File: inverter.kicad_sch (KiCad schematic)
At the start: 38 parts, among them IC3 L6498D, IC4 L6498D, IC5 L6498D, J2 43650-0303, J5 2159310271, Q1 IPD320N20N3GATMA1, Q2 IPD320N20N3GATMA1, Q3 IPD320N20N3GATMA1, Q4 IPD320N20N3GATMA1, Q5 IPD320N20N3GATMA1, Q6 IPD320N20N3GATMA1

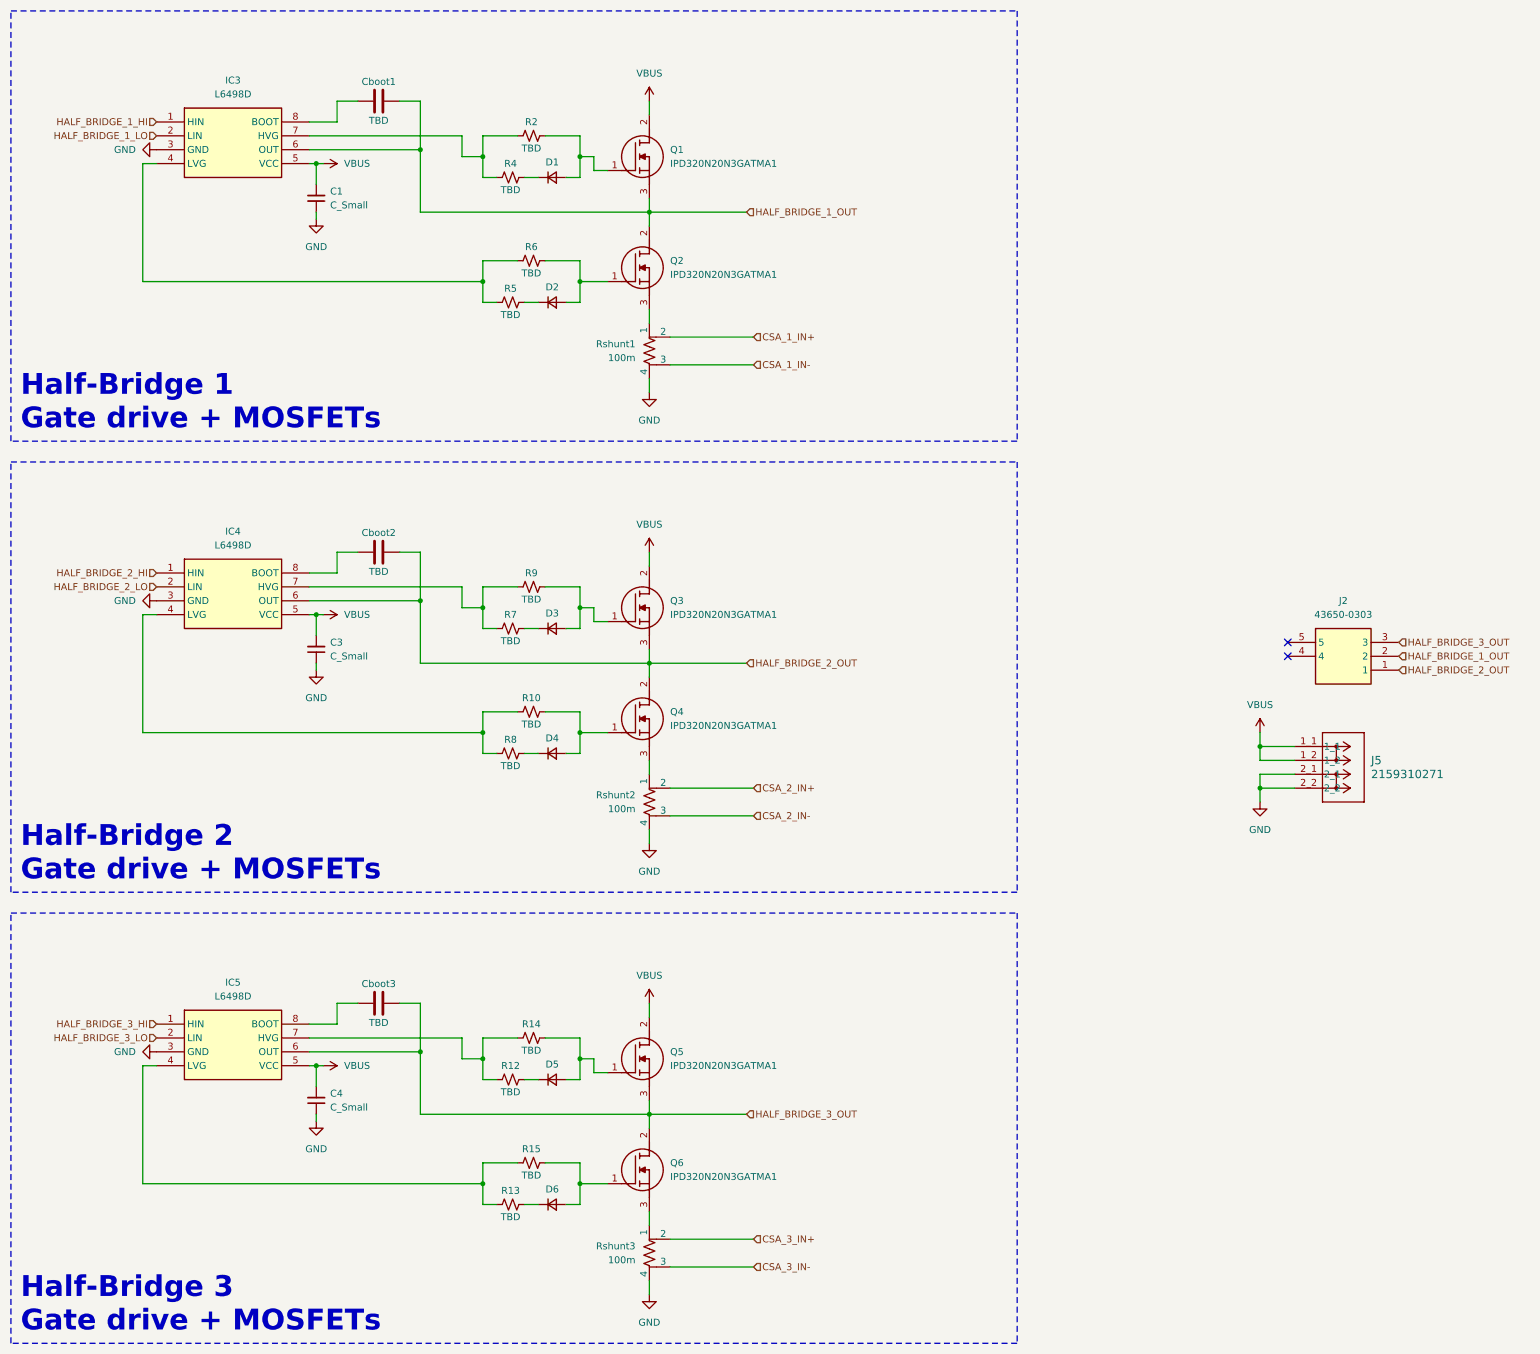
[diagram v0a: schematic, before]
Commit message: More routing
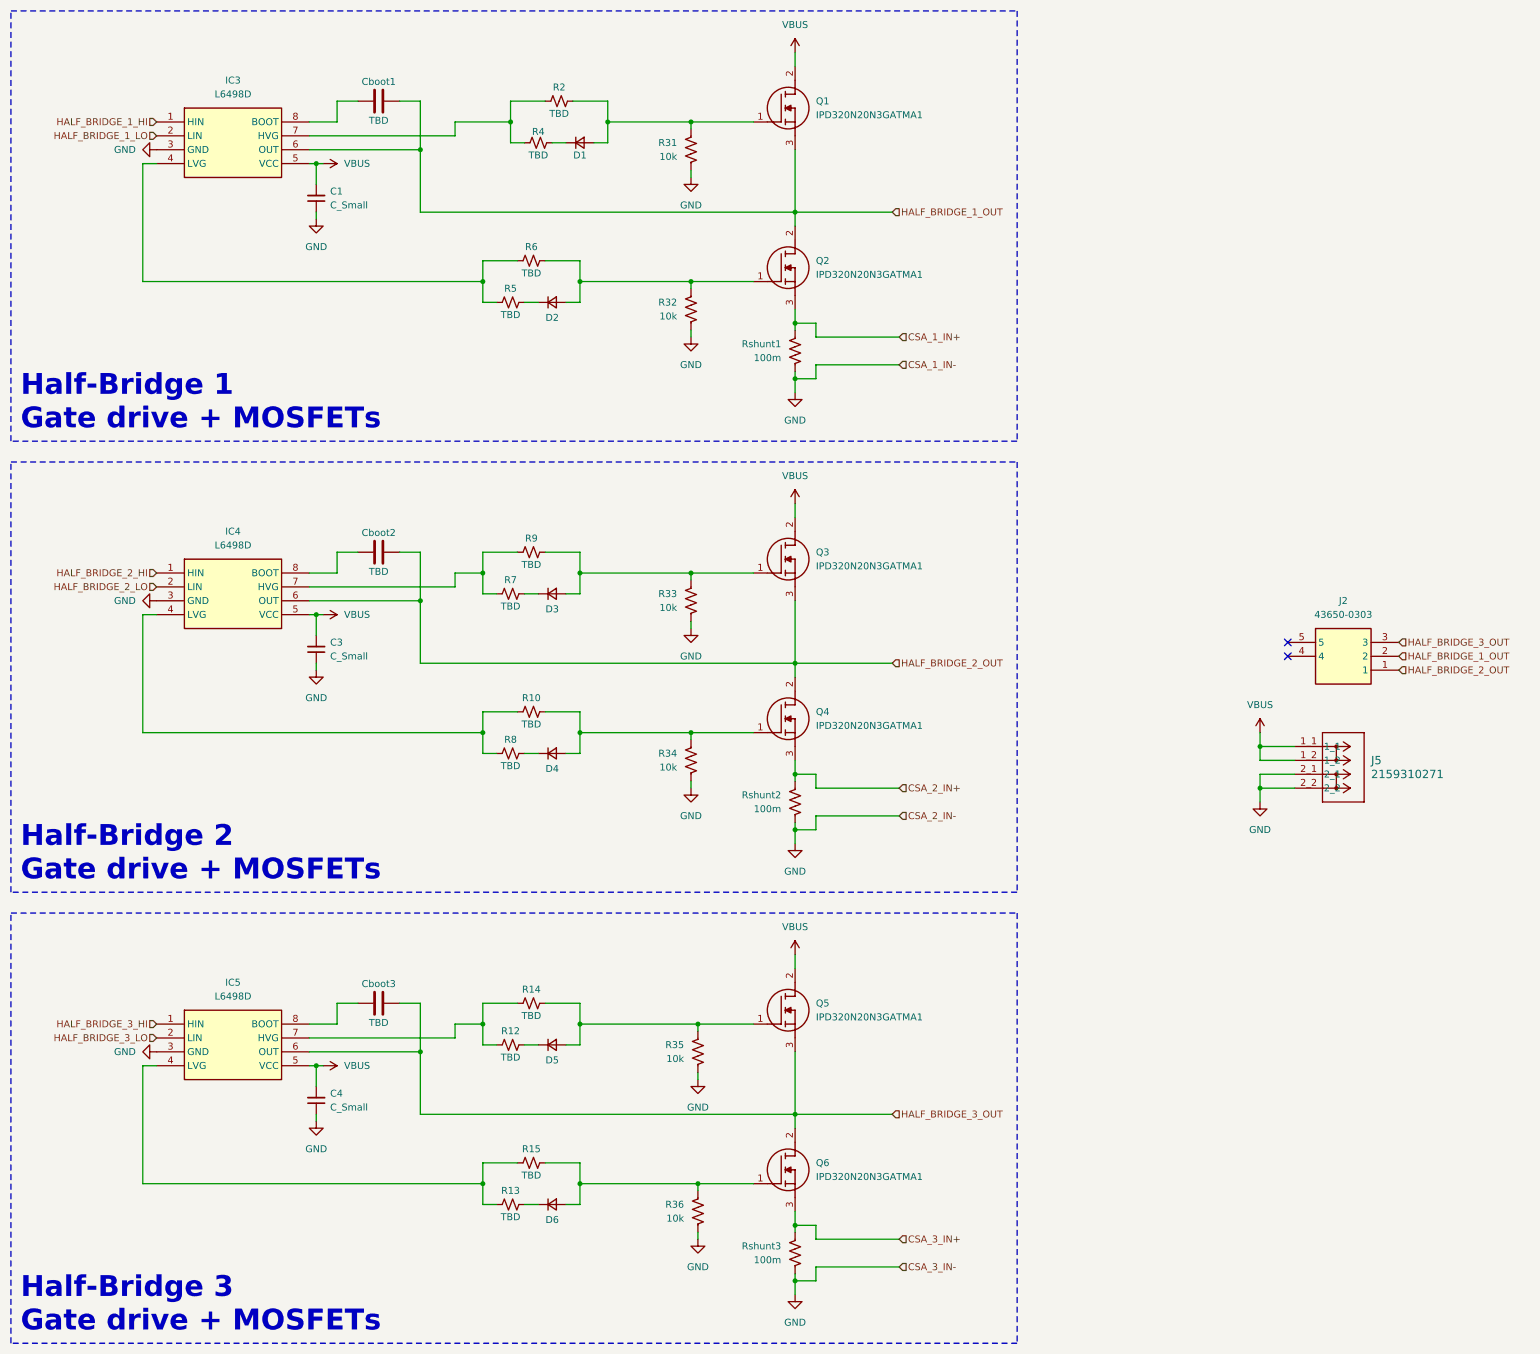
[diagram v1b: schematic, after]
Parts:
- removed Rshunt1, Rshunt2, Rshunt3: 100m, Resistor_SMD:R_0805_2012Metric, symbol Device:R_Shunt_US
- added R31, R32, R33, R34, R35, R36: 10k, Resistor_SMD:R_0603_1608Metric, symbol Device:R_US
- added Rshunt1, Rshunt2, Rshunt3: 100m, Resistor_SMD:R_1206_3216Metric, symbol Device:R_US
- D1, D2, D3, D4, D5, D6: footprint (none) -> Diode_SMD:D_0603_1608Metric
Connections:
- net CSA_1_IN+: now also Q2.3 (S), Rshunt1.1
- net CSA_2_IN+: now also Q4.3 (S), Rshunt2.1
- net CSA_3_IN+: now also Q6.3 (S), Rshunt3.1
- net GND: now also R31.2, R32.2, R33.2, R34.2, R35.2, R36.2, Rshunt1.2, Rshunt2.2, Rshunt3.2
- net at D1.2 (A), Q1.1 (G), R2.2: now also R31.1
- net at D3.2 (A), Q3.1 (G), R9.2: now also R33.1
- net at D2.2 (A), Q2.1 (G), R6.2: now also R32.1
- net at D6.2 (A), Q6.1 (G), R15.2: now also R36.1
- net at D4.2 (A), Q4.1 (G), R10.2: now also R34.1
- net at D5.2 (A), Q5.1 (G), R14.2: now also R35.1
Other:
- moved on the sheet: D1, D3, D5, Q1, Q2, Q3, Q4, Q5, Q6, R12, R14, R2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
